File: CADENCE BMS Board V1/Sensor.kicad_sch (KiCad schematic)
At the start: 65 parts, among them IC1 R5432V407BA, J1 Screw_Terminal_01x02, J21 Conn_01x02, Q1 P-Channel FET, Q10 N-MOS, Q2 60V Enhancement, Q3 60V Enhancement, Q4 60V Enhancement, Q5 Q_NMOS_DSG, Q6 Q_NMOS_DSG, Q7 Q_NMOS_DSG, Q8 N-MOS, Q9 N-MOS, U4 BQ34Z100-R2, U5 MCP9600-E_MX

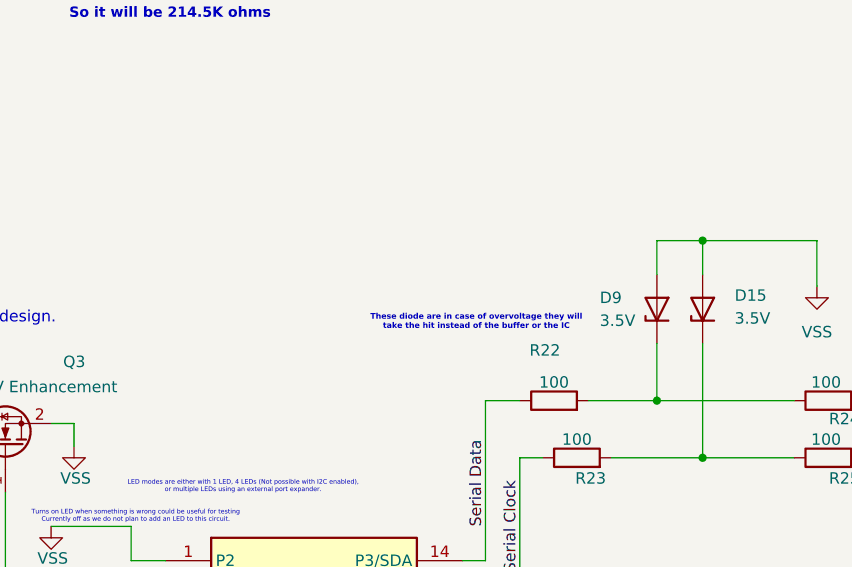
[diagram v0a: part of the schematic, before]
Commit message: Updates to component testing
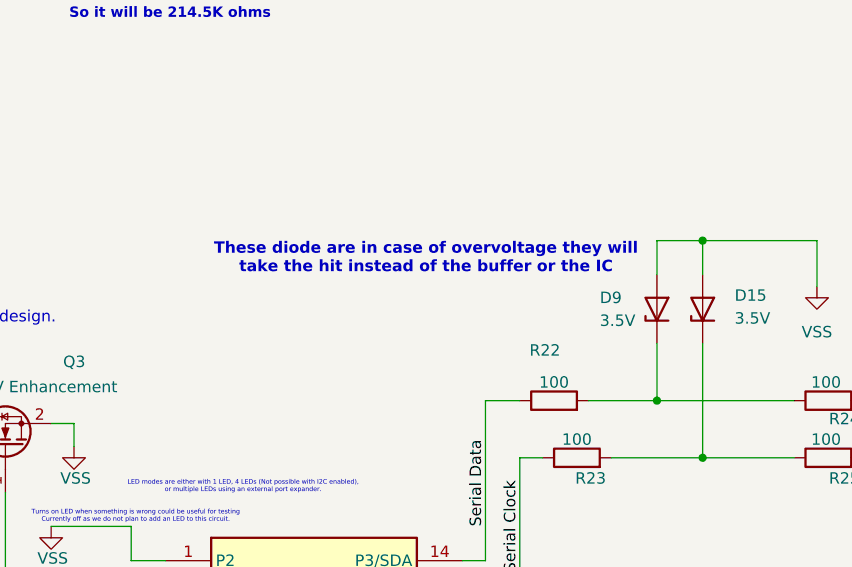
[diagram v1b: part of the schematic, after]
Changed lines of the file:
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@@
 	(text "These diode are in case of overvoltage they will\ntake the hit instead of the buffer or the IC"
 		(exclude_from_sim no)
-		(at 160.274 92.964 0)
+		(at 154.686 85.852 0)
 		(effects
 			(font
-				(size 0.635 0.635)
+				(size 1.27 1.27)
 				(thickness 0.127)
 				(bold yes)
